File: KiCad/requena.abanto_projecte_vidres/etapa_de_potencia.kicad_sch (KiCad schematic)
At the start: 9 parts, among them U1 VNH5019A-E

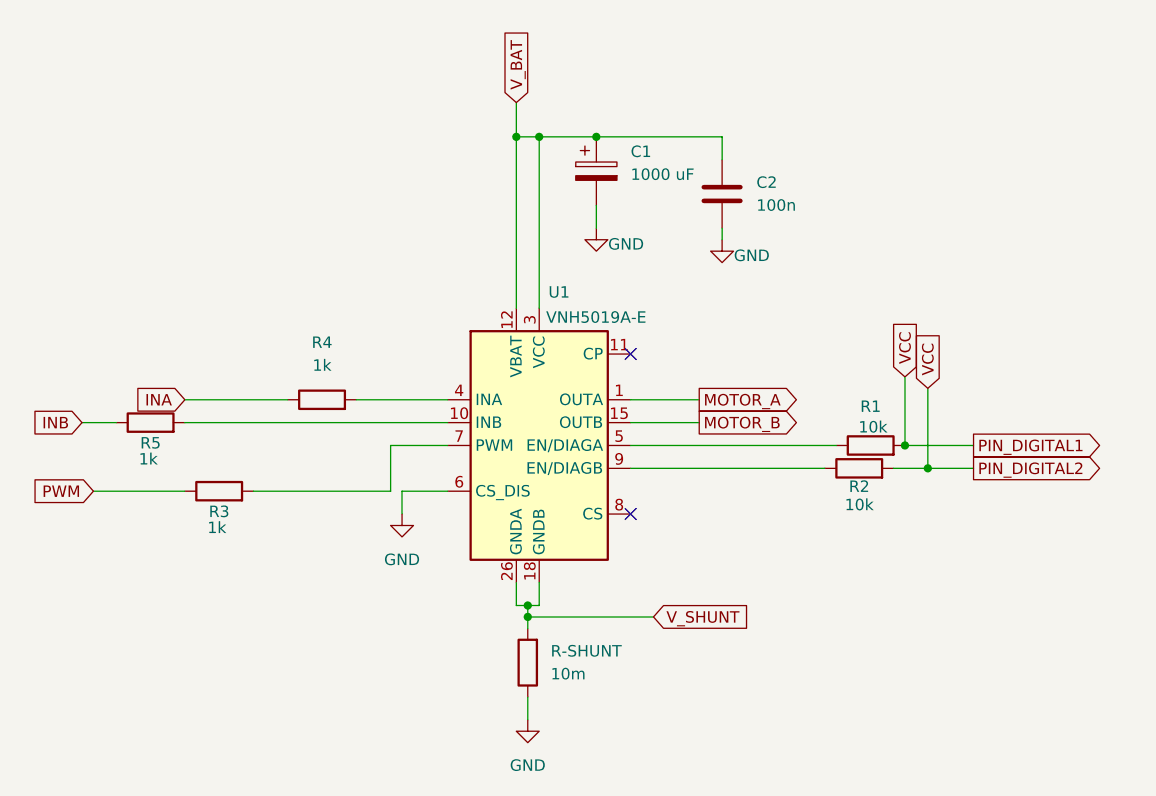
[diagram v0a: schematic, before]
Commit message: saywallahibro,canvis
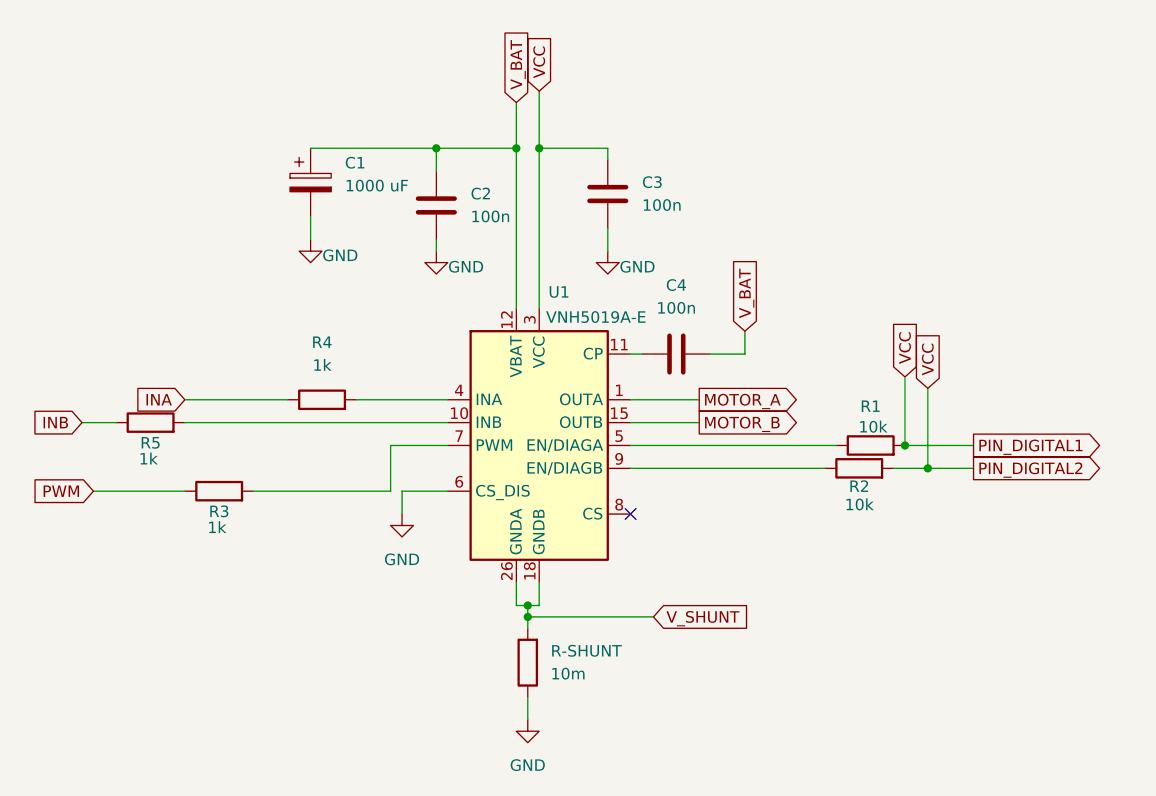
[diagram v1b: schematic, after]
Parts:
- added C3, C4: 100n, symbol Device:C
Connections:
- net GND: now also C3.2
- net PIN_DIGITAL1: now also U1.13 (VCC), U1.23 (VCC), U1.3 (VCC), U1.31 (VCC), C3.1
- net V_BAT: now also C4.2; no longer U1.13 (VCC), U1.23 (VCC), U1.3 (VCC), U1.31 (VCC)
- net at U1.11 (CP): now also C4.1
- no-connect marks 2 -> 1
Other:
- moved on the sheet: C1, C2
